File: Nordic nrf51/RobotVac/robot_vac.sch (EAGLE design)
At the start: 22 parts, among them IC4 317T, IC5 LM340H-05, J1 1X2-3.5MM, J2 ARDUINO_R3_SHIELDNOLABELS, X1 HD44780LCD-1602

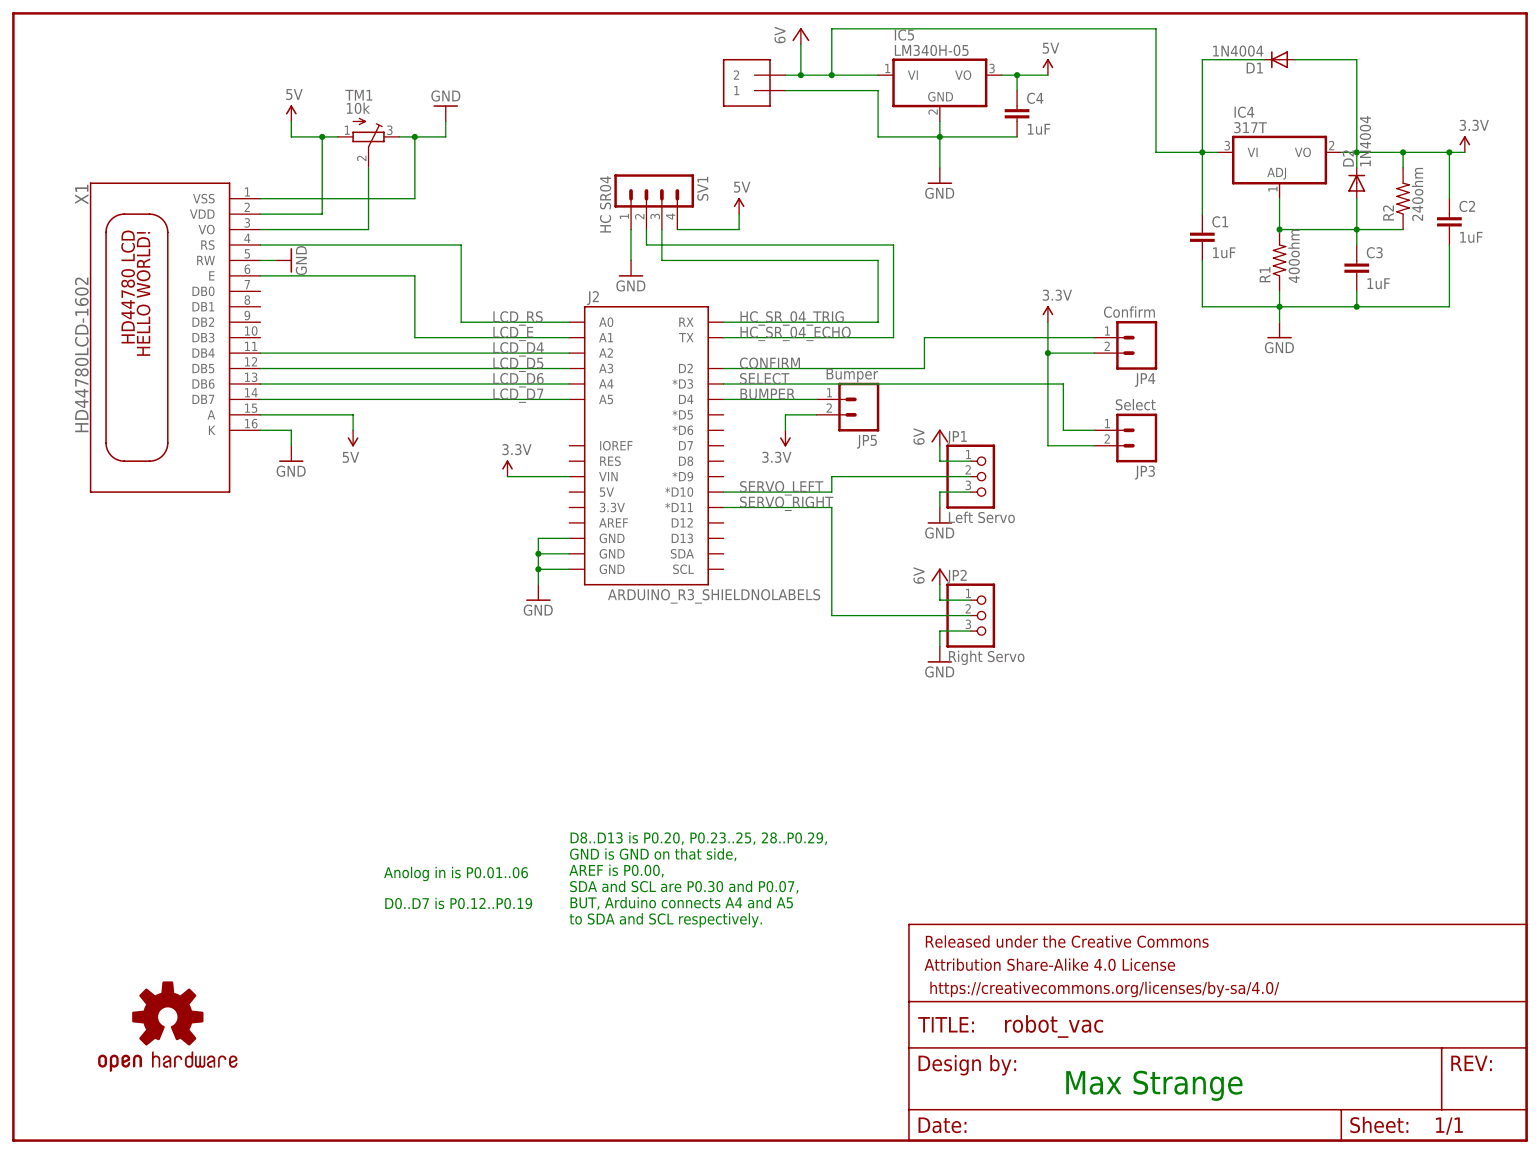
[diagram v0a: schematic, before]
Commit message: Update 1/26/16
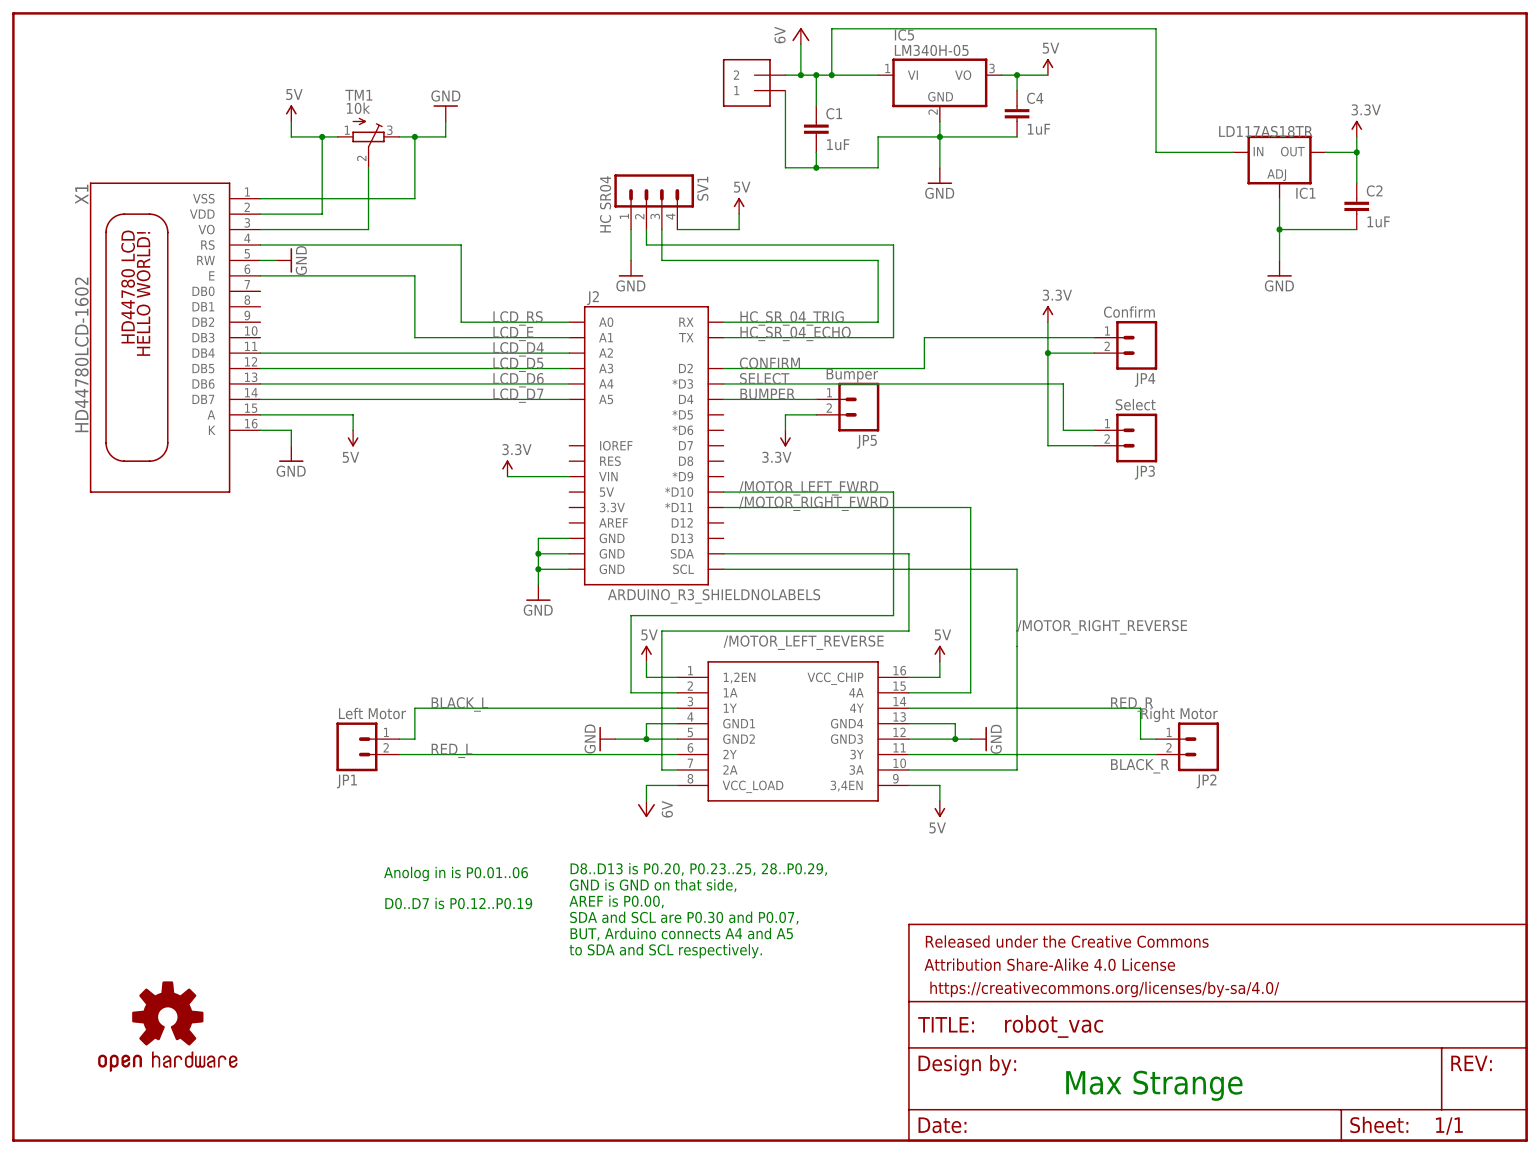
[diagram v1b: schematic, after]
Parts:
- removed C3: 1uF, SparkFun-Capacitors:CAPPTH
- removed D1, D2: 1N4004, adafruit:1N4004
- removed IC4: 317T, linear:317T
- removed R1: 400ohm, SparkFun-Passives:RESISTORPTH-1/2W
- removed R2: 240ohm, SparkFun-Passives:RESISTORPTH-1/2W
- added H_BRIDGE: SN75441_H_BRIDGE, max parts:SN75441_H_BRIDGE
- added IC1: LD117AS18TR, v-reg:LD117AS18TR
- JP1: value Left Servo -> Left Motor; device adafruit:PINHD-1X3 -> SparkFun-Connectors:M02LOCK
- JP2: value Right Servo -> Right Motor; device adafruit:PINHD-1X3 -> SparkFun-Connectors:M02LOCK
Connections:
- removed net N$3: C3.1, D2.A, IC4.ADJ, R1.2, R2.1
- removed net SERVO_LEFT: J2.*D10, JP1.2
- removed net SERVO_RIGHT: J2.*D11, JP2.2
- new net /MOTOR_LEFT_FWRD: H_BRIDGE.1A, J2.*D10
- new net /MOTOR_LEFT_REVERSE: H_BRIDGE.2A, J2.SDA
- new net /MOTOR_RIGHT_FWRD: H_BRIDGE.4A, J2.*D11
- new net /MOTOR_RIGHT_REVERSE: H_BRIDGE.3A, J2.SCL
- new net BLACK_L: H_BRIDGE.1Y, JP1.1
- new net BLACK_R: H_BRIDGE.3Y, JP2.2
- new net RED_L: H_BRIDGE.2Y, JP1.2
- new net RED_R: H_BRIDGE.4Y, JP2.1
- net 3.3V: now also IC1.OUT; no longer D1.A, D2.C, IC4.VO, R2.2
- net 5V: now also H_BRIDGE.1,2EN, H_BRIDGE.3,4EN, H_BRIDGE.VCC_CHIP
- net GND: now also H_BRIDGE.GND1, H_BRIDGE.GND2, H_BRIDGE.GND3, H_BRIDGE.GND4, IC1.ADJ; no longer C3.2, JP1.3, JP2.3, R1.1
- net VCC: now also H_BRIDGE.VCC_LOAD, IC1.IN; no longer D1.C, IC4.VI, JP1.1, JP2.1
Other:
- moved on the sheet: C1, C2
